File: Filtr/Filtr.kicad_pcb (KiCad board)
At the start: 2 copper layers, 80 x 50 mm, 40 parts, among them J1 Barrel_Jack_Switch, J2 Conn_01x04_Pin, SW3 RotaryEncoder_Switch, U1 TPS562200, U2 STM32G030K6Tx, U3 74HC595

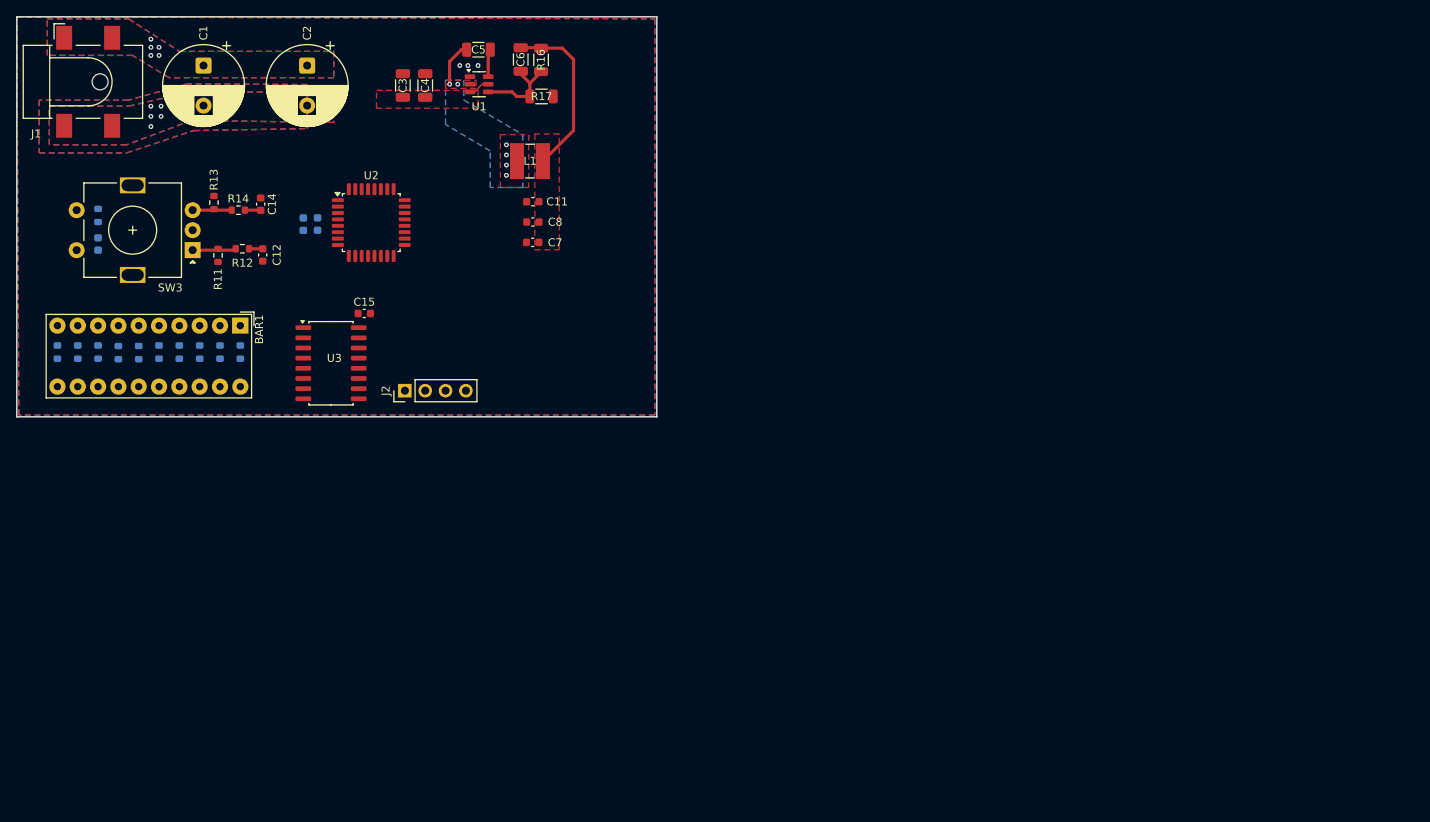
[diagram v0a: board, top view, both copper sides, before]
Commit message: Novy Design desky
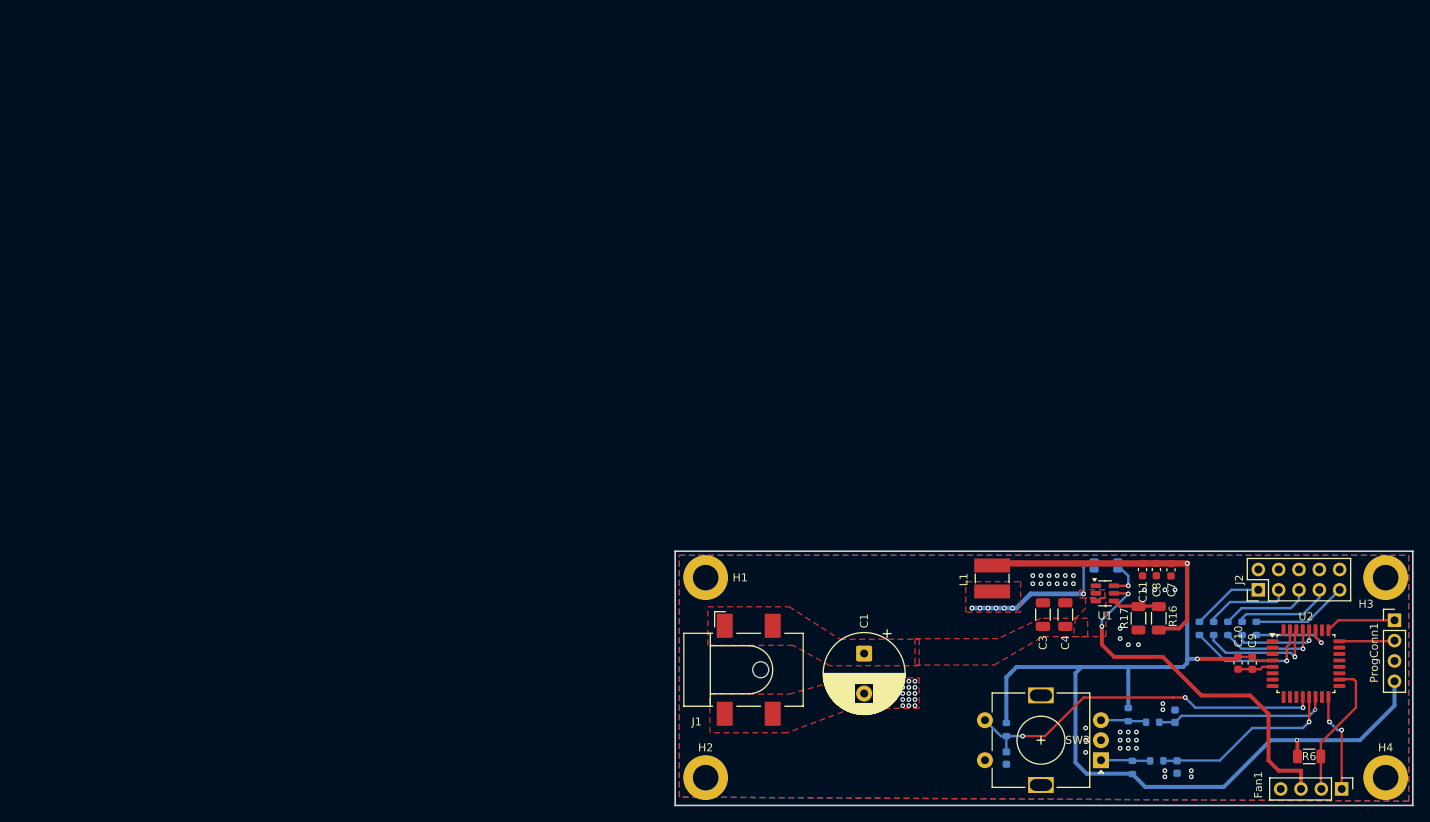
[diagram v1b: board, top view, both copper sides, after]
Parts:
- removed BAR1: HDSP-4830, Display:HDSP-4830
- removed C15: 0.1u, Capacitor_SMD:C_0603_1608Metric
- removed C2: C, Capacitor_THT:CP_Radial_D10.0mm_P5.00mm
- removed C6: C, Capacitor_SMD:C_1206_3216Metric
- removed R10, R7, R8, R9: R, Resistor_SMD:R_0603_1608Metric
- removed U3: 74HC595, Package_SO:SO-16_5.3x10.2mm_P1.27mm
- added H1: MountingHole_Pad, MountingHole:MountingHole_3.2mm_M3_DIN965_Pad, F.Cu at (169.9, 91.7)
- added H2: MountingHole_Pad, MountingHole:MountingHole_3.2mm_M3_DIN965_Pad, F.Cu at (169.9, 116.7)
- added H3: MountingHole_Pad, MountingHole:MountingHole_3.2mm_M3_DIN965_Pad, F.Cu at (254.9, 91.7)
- added H4: MountingHole_Pad, MountingHole:MountingHole_3.2mm_M3_DIN965_Pad, F.Cu at (254.9, 116.7)
- added J2: Conn_02x05_Odd_Even, Connector_PinHeader_2.54mm:PinHeader_2x05_P2.54mm_Vertical, F.Cu at (239.0, 93.2)
- added ProgConn1: Conn_01x04_Pin, Connector_PinHeader_2.54mm:PinHeader_1x04_P2.54mm_Vertical, F.Cu at (256.0, 97.0)
- C10, C9: moved to F.Cu
- C12, C14, C5, R11, R12, R13, R14: moved to B.Cu
- R6: footprint Resistor_SMD:R_0603_1608Metric -> Resistor_SMD:R_1206_3216Metric; moved to F.Cu
- moved R1 153.8 mm to (238.8, 98.0)
- moved R6 152.4 mm to (245.4, 114.0), turned to 0 degrees
- moved R2 149.6 mm to (237.0, 98.0)
- moved R3 145.4 mm to (235.2, 98.0)
- moved R4 141.2 mm to (233.4, 98.0)
- moved R5 137.0 mm to (231.6, 98.0)
- moved C12 131.0 mm to (228.9, 115.4)
- moved C14 131.0 mm to (228.6, 109.0)
- moved R11 131.0 mm to (223.3, 115.4)
- moved R12 131.0 mm to (226.3, 114.6)
- moved R13 131.0 mm to (222.8, 108.8)
- moved R14 131.0 mm to (225.8, 109.8)
- moved C9 130.7 mm to (238.3, 102.4)
- moved C13 130.5 mm to (207.5, 114.2)
- moved R15 130.5 mm to (207.5, 110.7)
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- renumbered J2 to Fan1
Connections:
- R6 pad 1: LED6 -> +3V3
- R6 pad 2: Net-(BAR1E-A) -> TACHO
- U2 pad 11: PWM -> unconnected-(U2-PA4-Pad11)
- U2 pad 16: unconnected-(U2-PB1-Pad16) -> PWM
- U2 pad 24: unconnected-(U2-PA13-Pad24) -> SWDIO
- U2 pad 25: unconnected-(U2-PA14-Pad25) -> SWCLK
- U2 pad 27: unconnected-(U2-PB3-Pad27) -> LED1
- U2 pad 28: unconnected-(U2-PB4-Pad28) -> LED2
- U2 pad 29: unconnected-(U2-PB5-Pad29) -> LED3
- U2 pad 30: unconnected-(U2-PB6-Pad30) -> LED4
- U2 pad 31: unconnected-(U2-PB7-Pad31) -> LED5
- U2 pad 7: SER -> unconnected-(U2-PA0-Pad7)
- U2 pad 8: SRCLK -> unconnected-(U2-PA1-Pad8)
- U2 pad 9: RCLK -> unconnected-(U2-PA2-Pad9)
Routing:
- net +3V3: track 21.5 -> 156.2 mm, vias 0 -> 3
- net BTN1: track 0.00 -> 46.4 mm, vias 0 -> 3
- net V+: track 2.67 -> 46.6 mm, vias 5 -> 2
- net ENC_A: track 1.72 -> 23.4 mm, vias 0 -> 1
- net ENC_B: track 1.98 -> 21.8 mm, vias 0 -> 1
- net TACHO: track 0.00 -> 17.5 mm
- net LED5: track 0.00 -> 16.3 mm, vias 0 -> 1
- net LED4: track 0.00 -> 15.1 mm, vias 0 -> 1
- net L1: track 5.58 -> 19.4 mm, vias 6 -> 7
- net PWM: track 0.00 -> 12.5 mm, vias 0 -> 2
- net LED3: track 0.00 -> 12.4 mm, vias 0 -> 1
- net Net-(J2-Pin_7): track 0.00 -> 12.2 mm
- net Net-(J2-Pin_9): track 0.00 -> 12.1 mm
- net Net-(J2-Pin_5): track 0.00 -> 11.3 mm
- net Net-(J2-Pin_3): track 0.00 -> 10.8 mm
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- removed copper zone on B.Cu, net (none)
- removed copper zone on F.Cu, net (none)
- removed copper zone on F.Cu, net +3V3
- removed copper zone on B.Cu, net L1
- removed copper zone on B.Cu, net V+
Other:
- board size 80 x 50 mm -> 92.2 x 31.8 mm
